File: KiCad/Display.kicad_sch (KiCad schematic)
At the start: 31 parts, among them J1 DC, J2 USB-C, M1 OLED1.5-RGB, U1 L86-M33, U2 ESP32-PICO-MINI-02, U3 FT231XQ, U4 LMR16006+FB, U5 QR

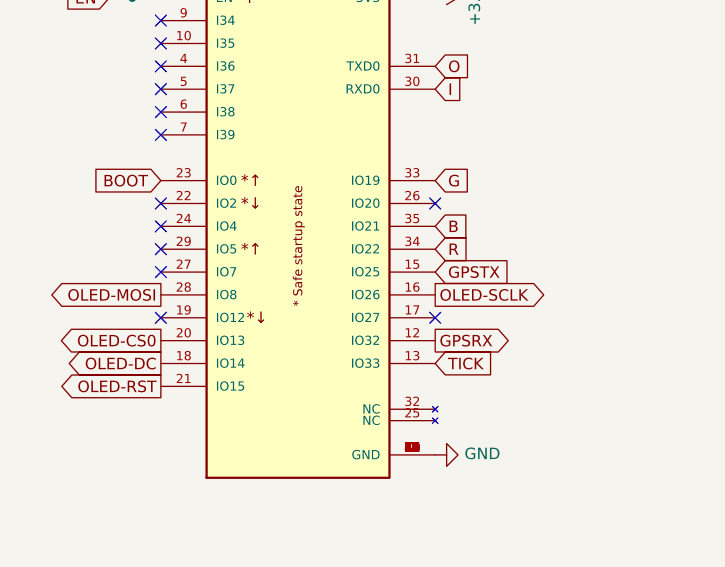
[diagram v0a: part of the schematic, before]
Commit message: tracked
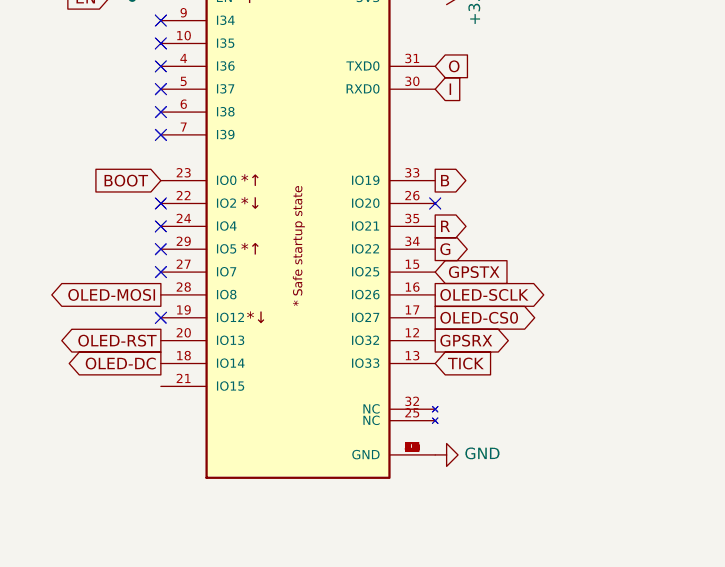
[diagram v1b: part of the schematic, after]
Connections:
- net B: now also U2.33 (IO19); no longer U2.35 (IO21)
- net G: now also U2.34 (IO22); no longer U2.33 (IO19)
- net OLED-CS0: now also U2.17 (IO27); no longer U2.20 (IO13)
- net OLED-RST: now also U2.20 (IO13); no longer U2.21 (IO15)
- net R: now also U2.35 (IO21); no longer U2.34 (IO22)
- no-connect marks 20 -> 19
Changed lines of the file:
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@@
   (no_connect (at 185.42 114.3))
   (no_connect (at 50.8 73.66))
-  (no_connect (at 81.28 83.82))
   (no_connect (at 48.26 139.7))
   (no_connect (at 48.26 142.24))
@@
     )
   )
-  (global_label "OLED-RST" (shape output) (at 50.8 91.44 180) (fields_autoplaced)
-    (effects (font (size 1.27 1.27)) (justify right))
-    (property "Intersheet References" "${INTERSHEET_REFS}" (id 0) (at 38.6787 91.3606 0)
+  (global_label "OLED-RST" (shape output) (at 50.8 86.36 180) (fields_autoplaced)
+    (effects (font (size 1.27 1.27)) (justify right))
+    (property "Intersheet References" "${INTERSHEET_REFS}" (id 0) (at 38.6787 86.2806 0)
       (effects (font (size 1.27 1.27)) (justify right) hide)
     )
@@
     )
   )
-  (global_label "R" (shape input) (at 81.28 76.2 0) (fields_autoplaced)
-    (effects (font (size 1.27 1.27)) (justify left))
-    (property "Intersheet References" "${INTERSHEET_REFS}" (id 0) (at -3.175 -16.51 0)
-      (effects (font (size 1.27 1.27)) hide)
+  (global_label "R" (shape output) (at 81.28 73.66 0) (fields_autoplaced)
+    (effects (font (size 1.27 1.27)) (justify left))
+    (property "Intersheet References" "${INTERSHEET_REFS}" (id 0) (at 84.8742 73.5806 0)
+      (effects (font (size 1.27 1.27)) (justify left) hide)
     )
   )
@@
     )
   )
-  (global_label "OLED-CS0" (shape output) (at 50.8 86.36 180) (fields_autoplaced)
-    (effects (font (size 1.27 1.27)) (justify right))
-    (property "Intersheet References" "${INTERSHEET_REFS}" (id 0) (at 38.4368 86.2806 0)
-      (effects (font (size 1.27 1.27)) (justify right) hide)
+  (global_label "OLED-CS0" (shape output) (at 81.28 83.82 0) (fields_autoplaced)
+    (effects (font (size 1.27 1.27)) (justify left))
+    (property "Intersheet References" "${INTERSHEET_REFS}" (id 0) (at 93.6432 83.8994 0)
+      (effects (font (size 1.27 1.27)) (justify left) hide)
     )
   )
@@
     )
   )
-  (global_label "G" (shape input) (at 81.28 68.58 0) (fields_autoplaced)
-    (effects (font (size 1.27 1.27)) (justify left))
-    (property "Intersheet References" "${INTERSHEET_REFS}" (id 0) (at -3.175 -19.05 0)
-      (effects (font (size 1.27 1.27)) hide)
+  (global_label "G" (shape output) (at 81.28 76.2 0) (fields_autoplaced)
+    (effects (font (size 1.27 1.27)) (justify left))
+    (property "Intersheet References" "${INTERSHEET_REFS}" (id 0) (at 84.8742 76.1206 0)
+      (effects (font (size 1.27 1.27)) (justify left) hide)
     )
   )
@@
     )
   )
-  (global_label "B" (shape input) (at 81.28 73.66 0) (fields_autoplaced)
-    (effects (font (size 1.27 1.27)) (justify left))
-    (property "Intersheet References" "${INTERSHEET_REFS}" (id 0) (at -3.175 -21.59 0)
-      (effects (font (size 1.27 1.27)) hide)
-    )
-  )
+  (global_label "B" (shape output) (at 81.28 68.58 0) (fields_autoplaced)
+    (effects (font (size 1.27 1.27)) (justify left))
+    (property "Intersheet References" "${INTERSHEET_REFS}" (id 0) (at 84.8742 68.5006 0)
+      (effects (font (size 1.27 1.27)) (justify left) hide)
+    )
+  )
